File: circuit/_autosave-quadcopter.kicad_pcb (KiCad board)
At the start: 4 copper layers, 37.7 x 37.7 mm, 111 parts, among them J1 Conn_01x01_Female, J10 Conn_01x01_Female, J11 Conn_01x01_Female, J12 Conn_01x01_Female, J13 Conn_01x01_Female, J14 Conn_01x01_Female, J15 Conn_01x01_Female, J16 Conn_01x01_Female, J17 Conn_01x01_Female, J18 USB_C_Receptacle_USB2.0, J19 Conn_01x08_Male, J2 Conn_01x01_Female, J20 Conn_01x04_Male, J21 Conn_01x01_Female, J22 Conn_01x01_Female, J23 Conn_01x01_Female, J24 Conn_01x01_Female, J25 Conn_01x01_Female, J26 Conn_01x01_Female, J27 Conn_01x01_Female, J28 Conn_01x01_Female, J29 Conn_01x01_Female, J3 Conn_01x01_Female, J30 Conn_01x01_Female, J31 Conn_01x01_Female, J32 Conn_01x01_Female, J33 Conn_01x01_Female, J34 Conn_01x01_Female, J36 Conn_01x01_Female, J37 Conn_01x01_Female, J38 Conn_01x01_Female, J39 Conn_01x01_Female, J4 Conn_01x01_Female, J40 Conn_01x01_Female, J41 Conn_01x01_Female, J42 Conn_01x01_Female, J43 Conn_01x01_Female, J44 Conn_01x01_Female, J45 Conn_01x01_Female, J46 Conn_01x01_Female, J47 Conn_01x01_Female, J48 Conn_01x01_Female, J49 Conn_01x01_Female, J5 Conn_01x01_Female, J50 Conn_01x01_Female, J51 Conn_01x01_Female, J6 Conn_01x01_Female, J7 Conn_01x01_Female, J8 Conn_01x01_Female, J9 Conn_01x01_Female, SW1 SW_DIP_x01, U1 STM32G431CBU6, U2 ICM-42605, U3 DPS310, U4 3V3, U5 5V, U6 AT7456E, U7 W25Q128JVS, Y1 16M, Y2 27M

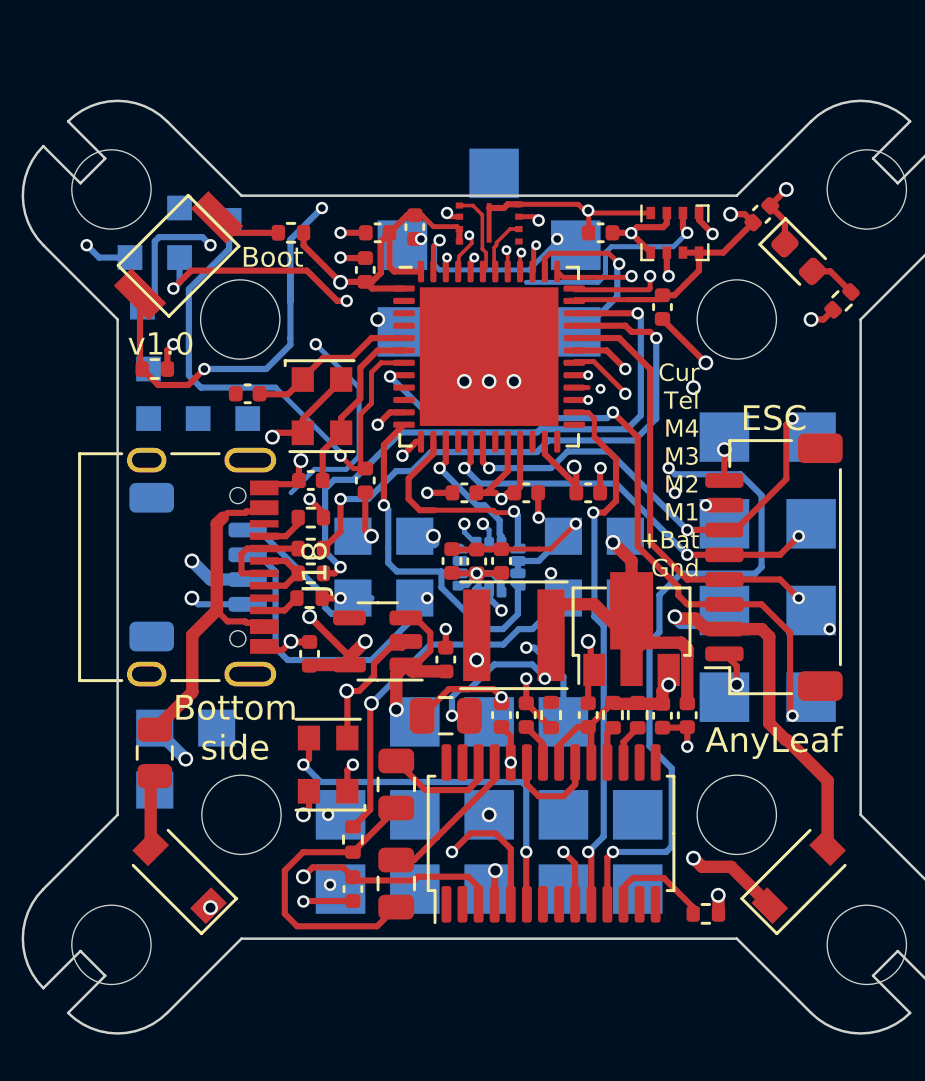
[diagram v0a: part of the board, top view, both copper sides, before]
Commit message: More work on CRSF
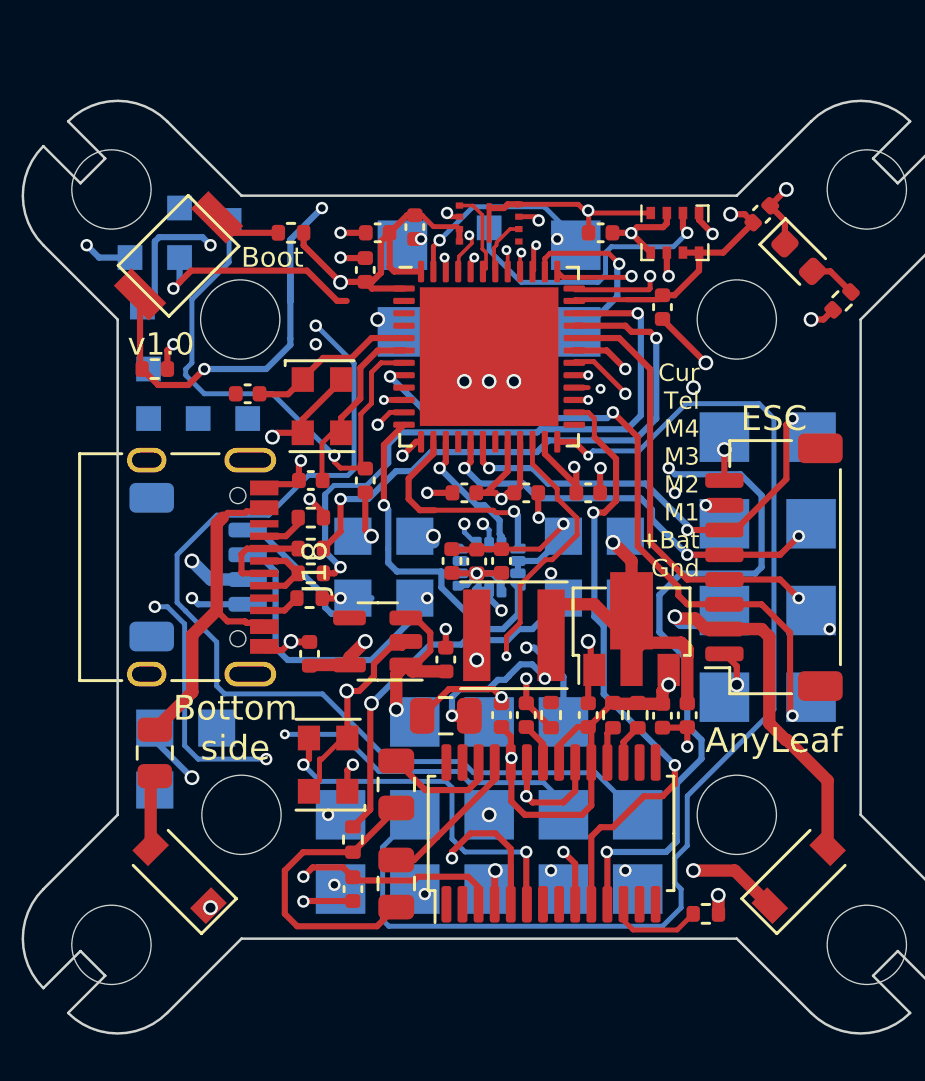
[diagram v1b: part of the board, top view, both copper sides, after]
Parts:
- J50: footprint TestPoint:TestPoint_Pad_2.0x2.0mm -> TestPoint:TestPoint_Pad_1.0x1.0mm
- moved J50 2.21 mm to (137.0, 73.8)
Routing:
- net /UART3_RX: track 0.00 -> 48.9 mm, vias 0 -> 1
- net /UART1_RX: track 12.5 -> 52.6 mm, vias 1 -> 2
- net /UART1_TX: track 17.2 -> 53.8 mm, vias 2 -> 5
- net /UART2_TX: track 0.00 -> 34.3 mm, vias 0 -> 2
- net GND: track 69.0 -> 103.1 mm
- net /UART2_RX: track 1.27 -> 28.7 mm, vias 1 -> 2
- net /UART3_TX: track 0.00 -> 25.0 mm, vias 0 -> 2
- net /SWDIO: track 29.1 -> 8.98 mm
- net +5V: track 27.6 -> 46.3 mm
- net /SWCLK: track 24.3 -> 12.5 mm, vias 3 -> 2
- net +3V3: track 66.8 -> 76.5 mm, vias 13 -> 12
- net /SCK_2: track 22.1 -> 25.1 mm
- net /SDA2: track 19.3 -> 22.3 mm
- net Net-(D2-Pad1): track 18.3 -> 20.3 mm
- net /UART4_RX: track 28.9 -> 29.8 mm
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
